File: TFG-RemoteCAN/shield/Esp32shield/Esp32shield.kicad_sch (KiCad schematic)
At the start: 8 parts, among them J1 PINS_1, J2 PINS_2, J3 Screw_Terminal_01x02, J4 Conn_01x04, J5 Conn_01x01, J6 Conn_01x01, J7 Conn_01x01, J8 Conn_01x01

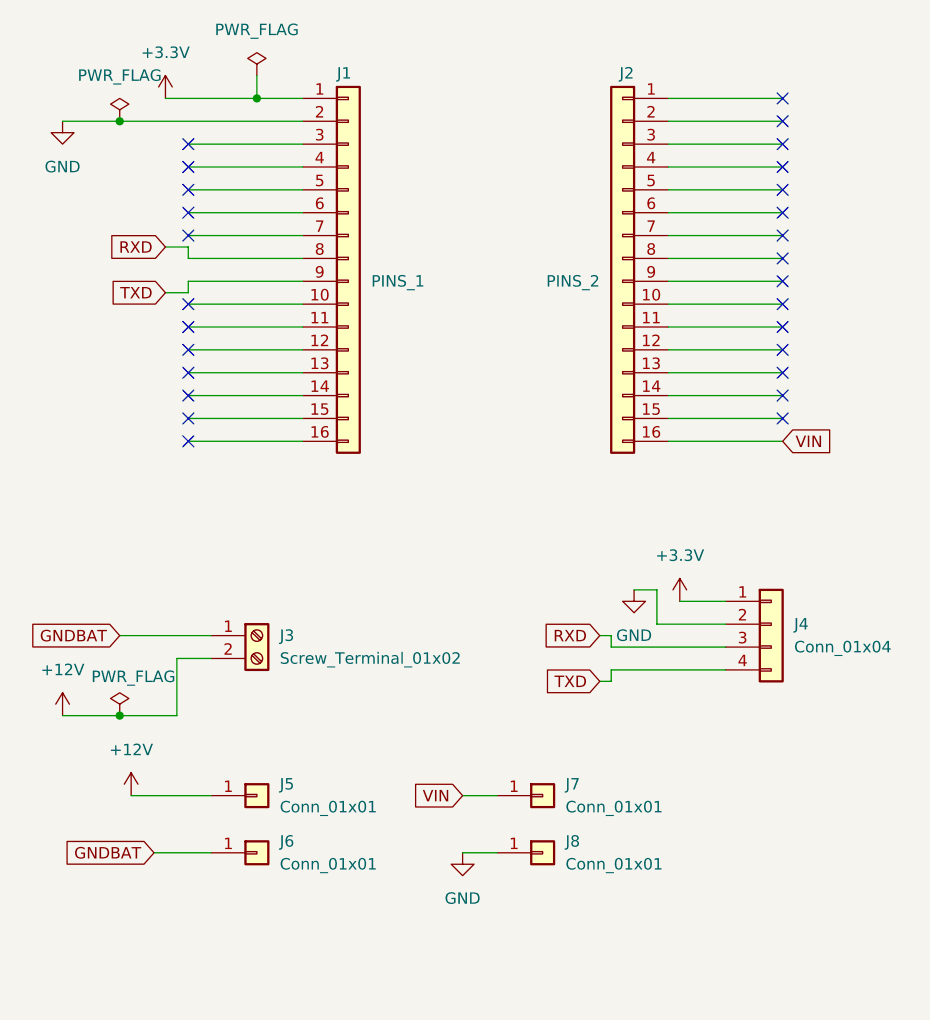
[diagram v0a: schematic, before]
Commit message: Versió 1.1
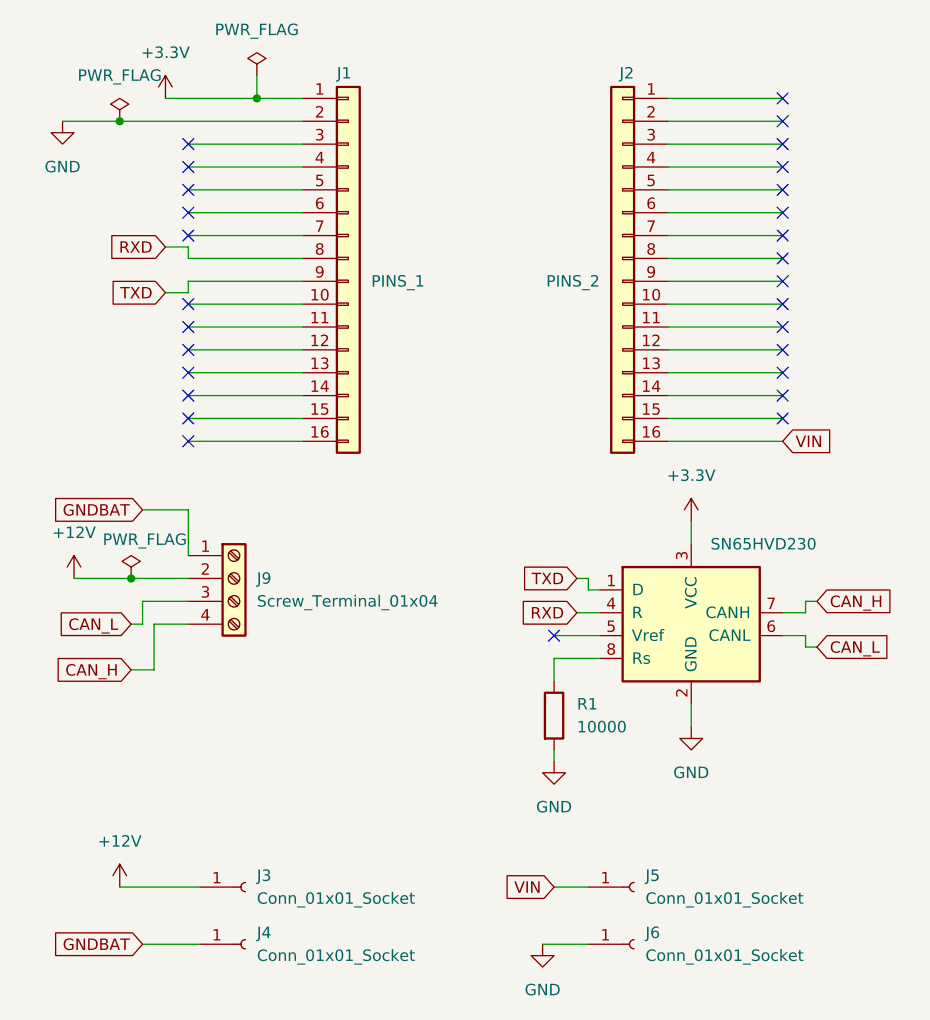
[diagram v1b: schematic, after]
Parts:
- removed J3: Screw_Terminal_01x02, TerminalBlock_Phoenix:TerminalBlock_Phoenix_MPT-0,5-2-2.54_1x02_P2.54mm_Horizontal, symbol Connector:Screw_Terminal_01x02
- removed J4: Conn_01x04, Connector_PinSocket_2.54mm:PinSocket_1x04_P2.54mm_Vertical, symbol Connector_Generic:Conn_01x04
- removed J5, J6, J7, J8: Conn_01x01, Connector_PinSocket_2.54mm:PinSocket_1x01_P2.54mm_Vertical, symbol Connector_Generic:Conn_01x01
- added J3, J4, J5, J6: Conn_01x01_Socket, MountingHole:MountingHole_2.2mm_M2_DIN965_Pad, symbol Connector:Conn_01x01_Socket
- added J9: Screw_Terminal_01x04, TerminalBlock_Phoenix:TerminalBlock_Phoenix_MPT-0,5-4-2.54_1x04_P2.54mm_Horizontal, symbol Connector:Screw_Terminal_01x04
- added R1: 10000, Resistor_THT:R_Axial_DIN0207_L6.3mm_D2.5mm_P7.62mm_Horizontal, symbol Device:R
- added U1: SN65HVD230, Package_SO:SOIC-8_3.9x4.9mm_P1.27mm, symbol Interface_CAN_LIN:SN65HVD230
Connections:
- net +12V: now also J3.1 (Pin_1), J9.2 (Pin_2)
- net +3.3V: now also U1.3 (VCC)
- net GND: now also J6.1 (Pin_1), R1.2, U1.2 (GND)
- net GNDBAT: now also J4.1 (Pin_1), J9.1 (Pin_1)
- net RXD: now also U1.4 (R)
- net TXD: now also U1.1 (D)
- net VIN: now also J5.1 (Pin_1)
- new net: R1.1, U1.8 (Rs)
- new net CAN_H: J9.4 (Pin_4), U1.7 (CANH)
- new net CAN_L: J9.3 (Pin_3), U1.6 (CANL)
- no-connect marks 27 -> 28
